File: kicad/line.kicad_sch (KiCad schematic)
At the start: 54 parts, among them J3 AudioJack3_Switch, J4 AudioJack3_Switch, Q3 2N7002, Q4 2N7002, SW12 RotaryEncoder, U12 OPA1637, U13 OPA1637

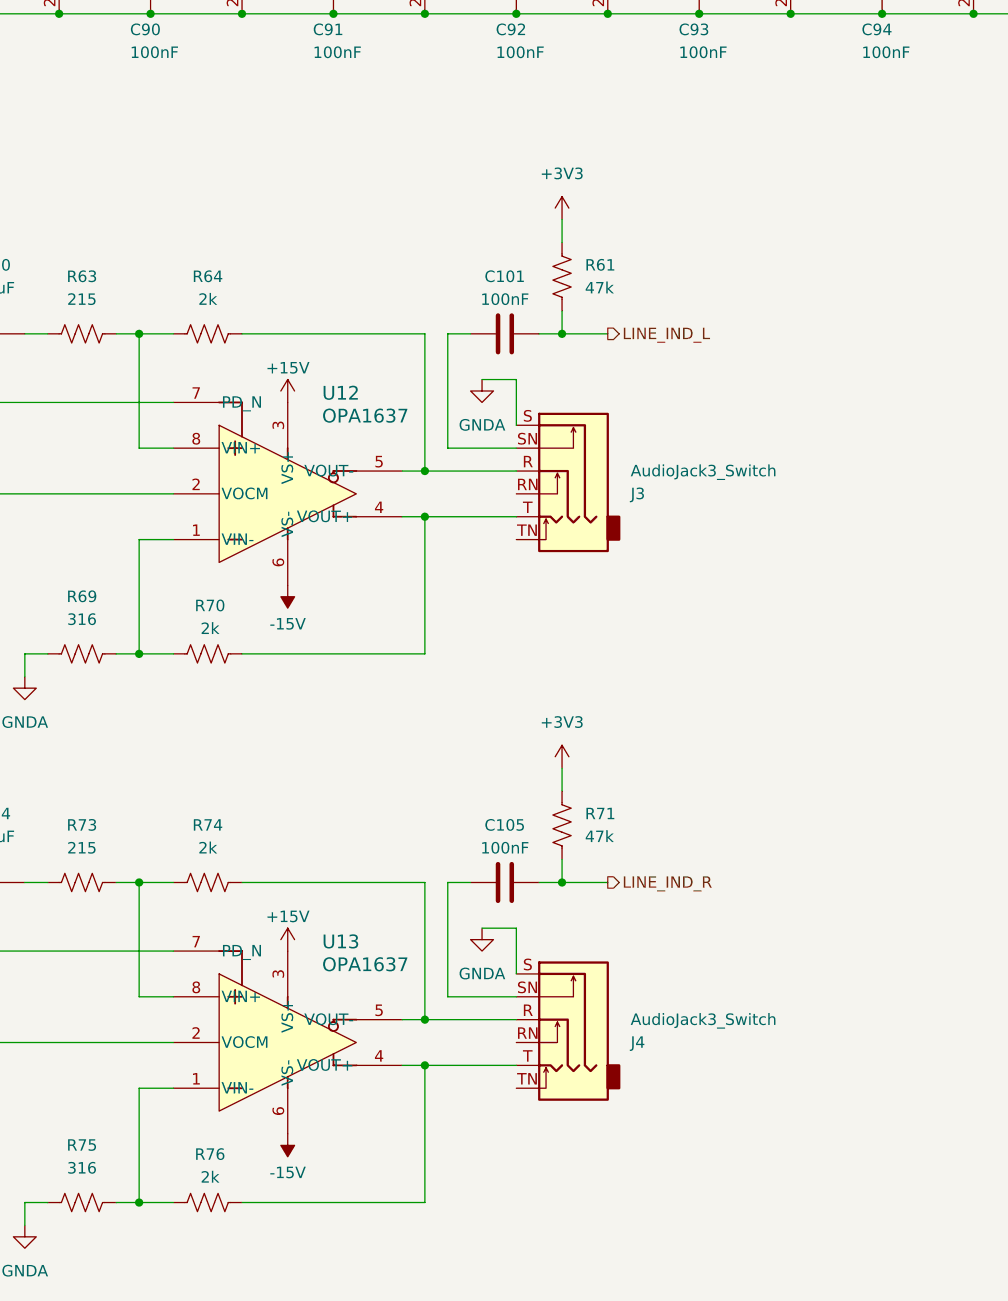
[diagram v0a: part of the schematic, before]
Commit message: bypass caps
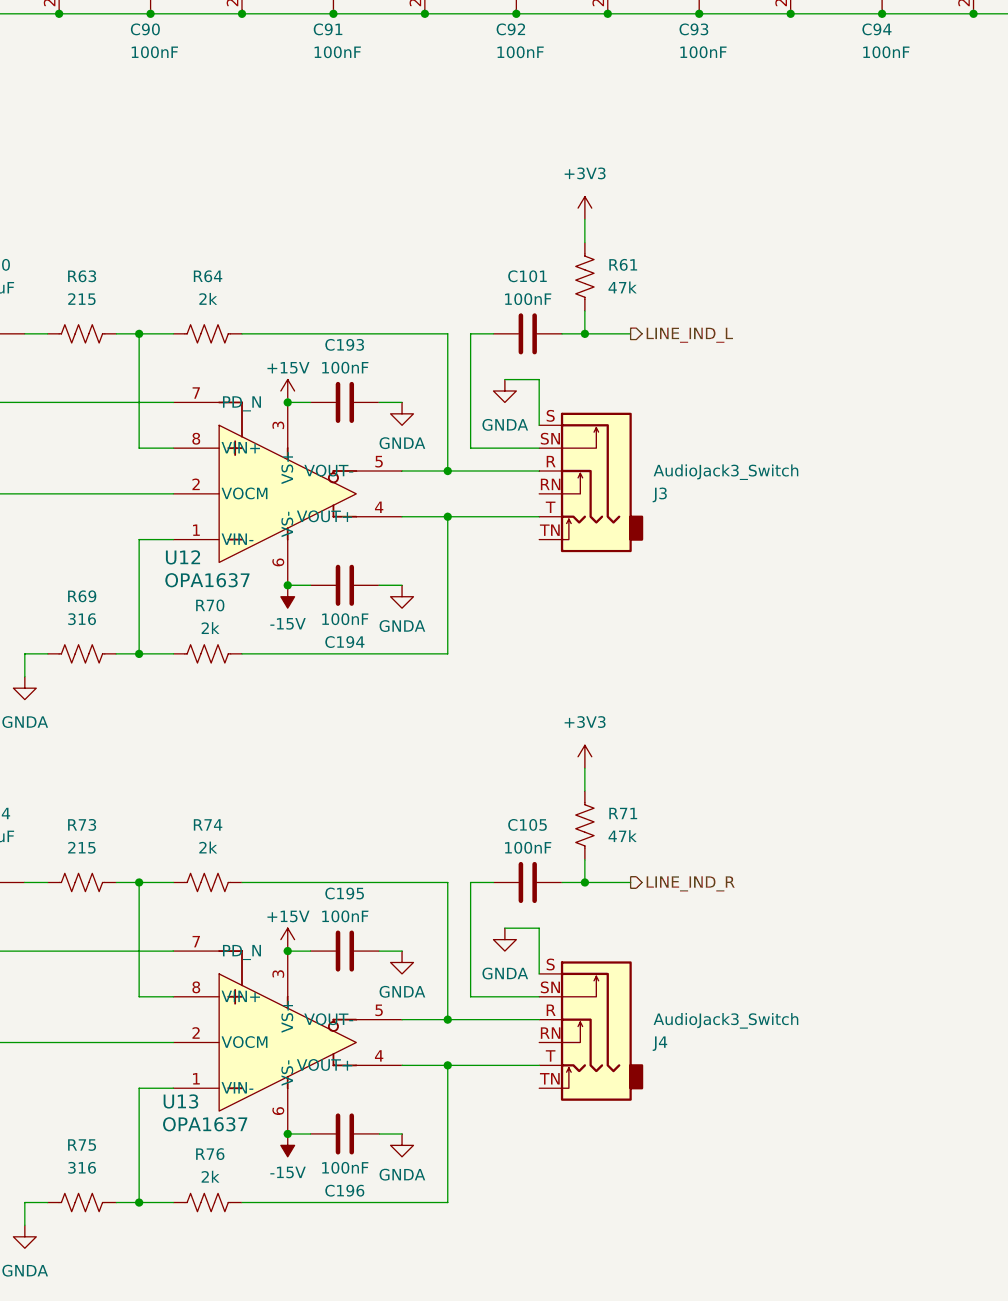
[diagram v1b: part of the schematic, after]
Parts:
- added C193, C194, C195, C196: 100nF, symbol Device:C
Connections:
- net +15V: now also C193.1, C195.1
- net -15V: now also C194.1, C196.1
- net GNDA: now also C193.2, C194.2, C195.2, C196.2
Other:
- moved on the sheet: C101, C105, J3, J4, R61, R71
